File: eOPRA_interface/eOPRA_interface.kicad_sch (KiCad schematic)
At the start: 23 parts, among them J1 CONN_01X02_MALE, J2 CONN_01X04_MALE, J3 CONN_01X04_MALE, J4 CONN_01X02_MALE, J5 CONN_01X03_MALE, J7 header_01x02, J8 CONN_01X04_MALE, Q4 Q_PMOS_DGS, U1 ARM-SWD-10, U10 USB_C_2.0, U27 Mounting-holes, U28 Mounting-holes, U5 XT-X, U7 Mounting-holes, U8 Mounting-holes

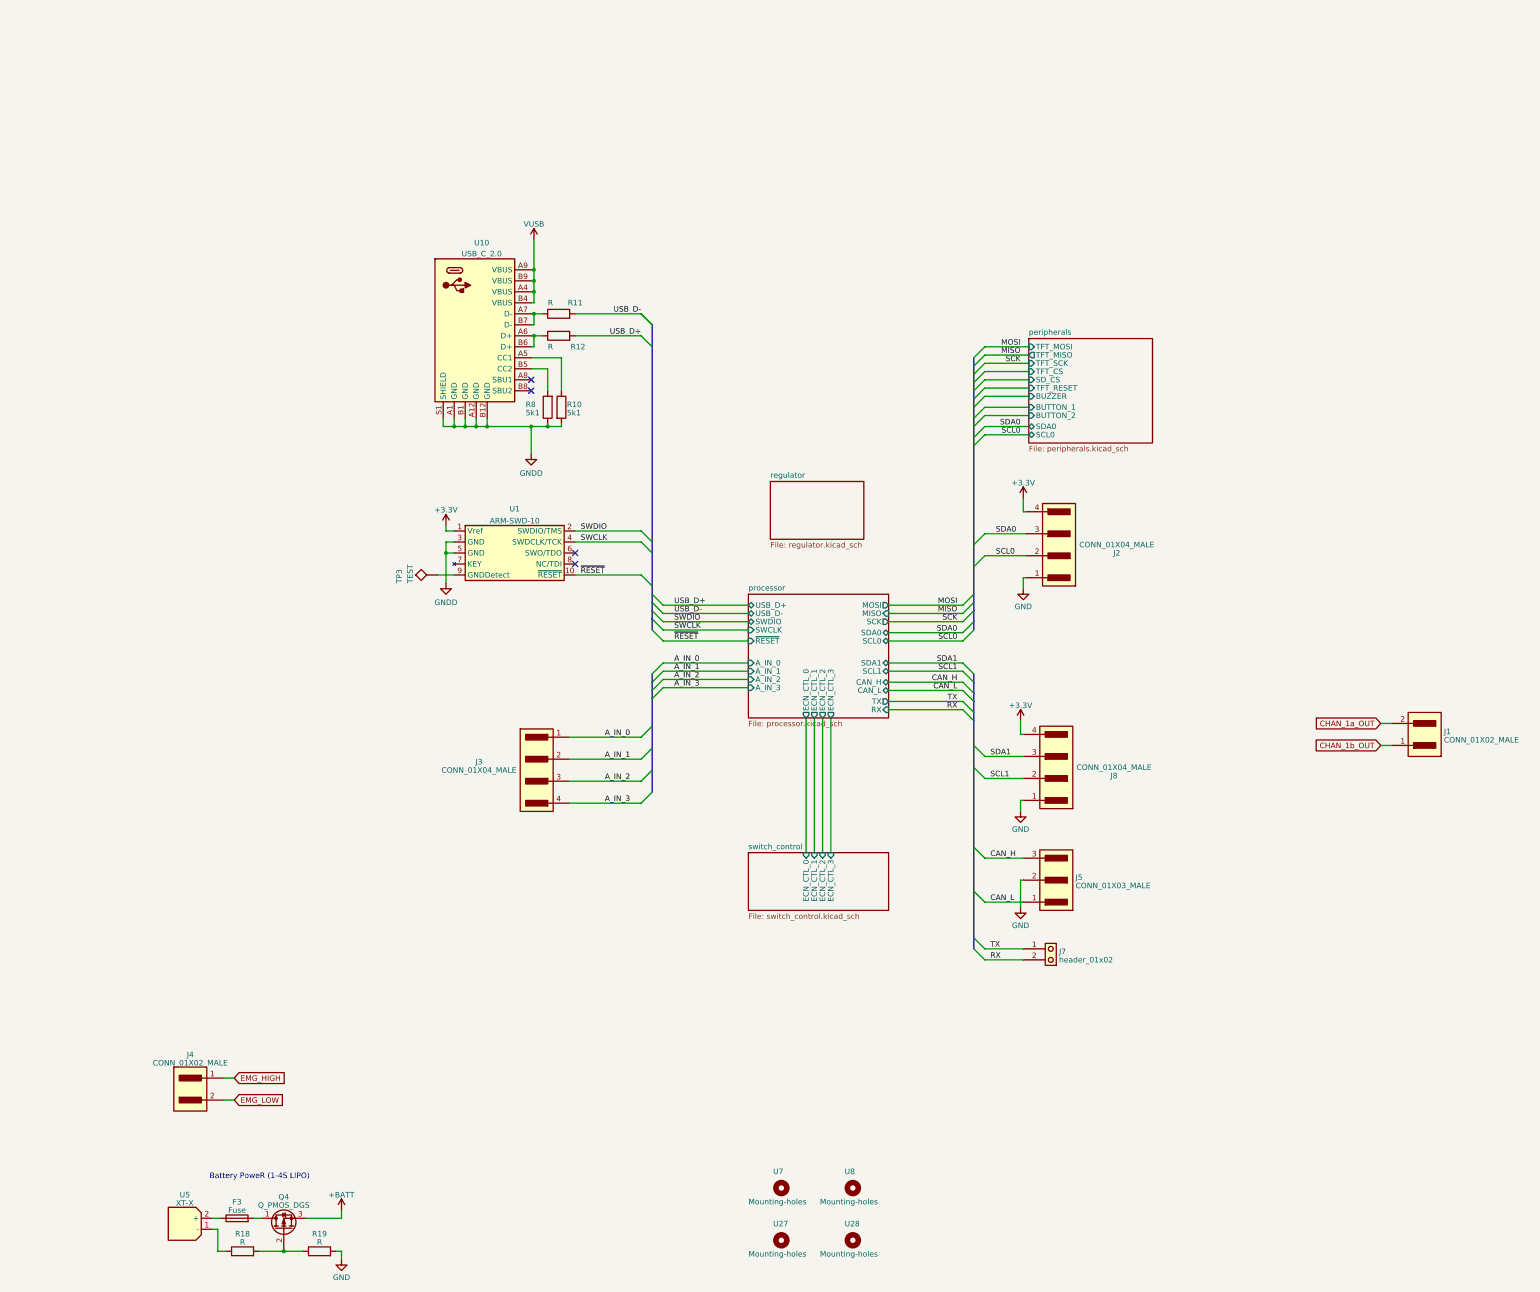
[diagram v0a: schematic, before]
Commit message: schematic v1.0 finished
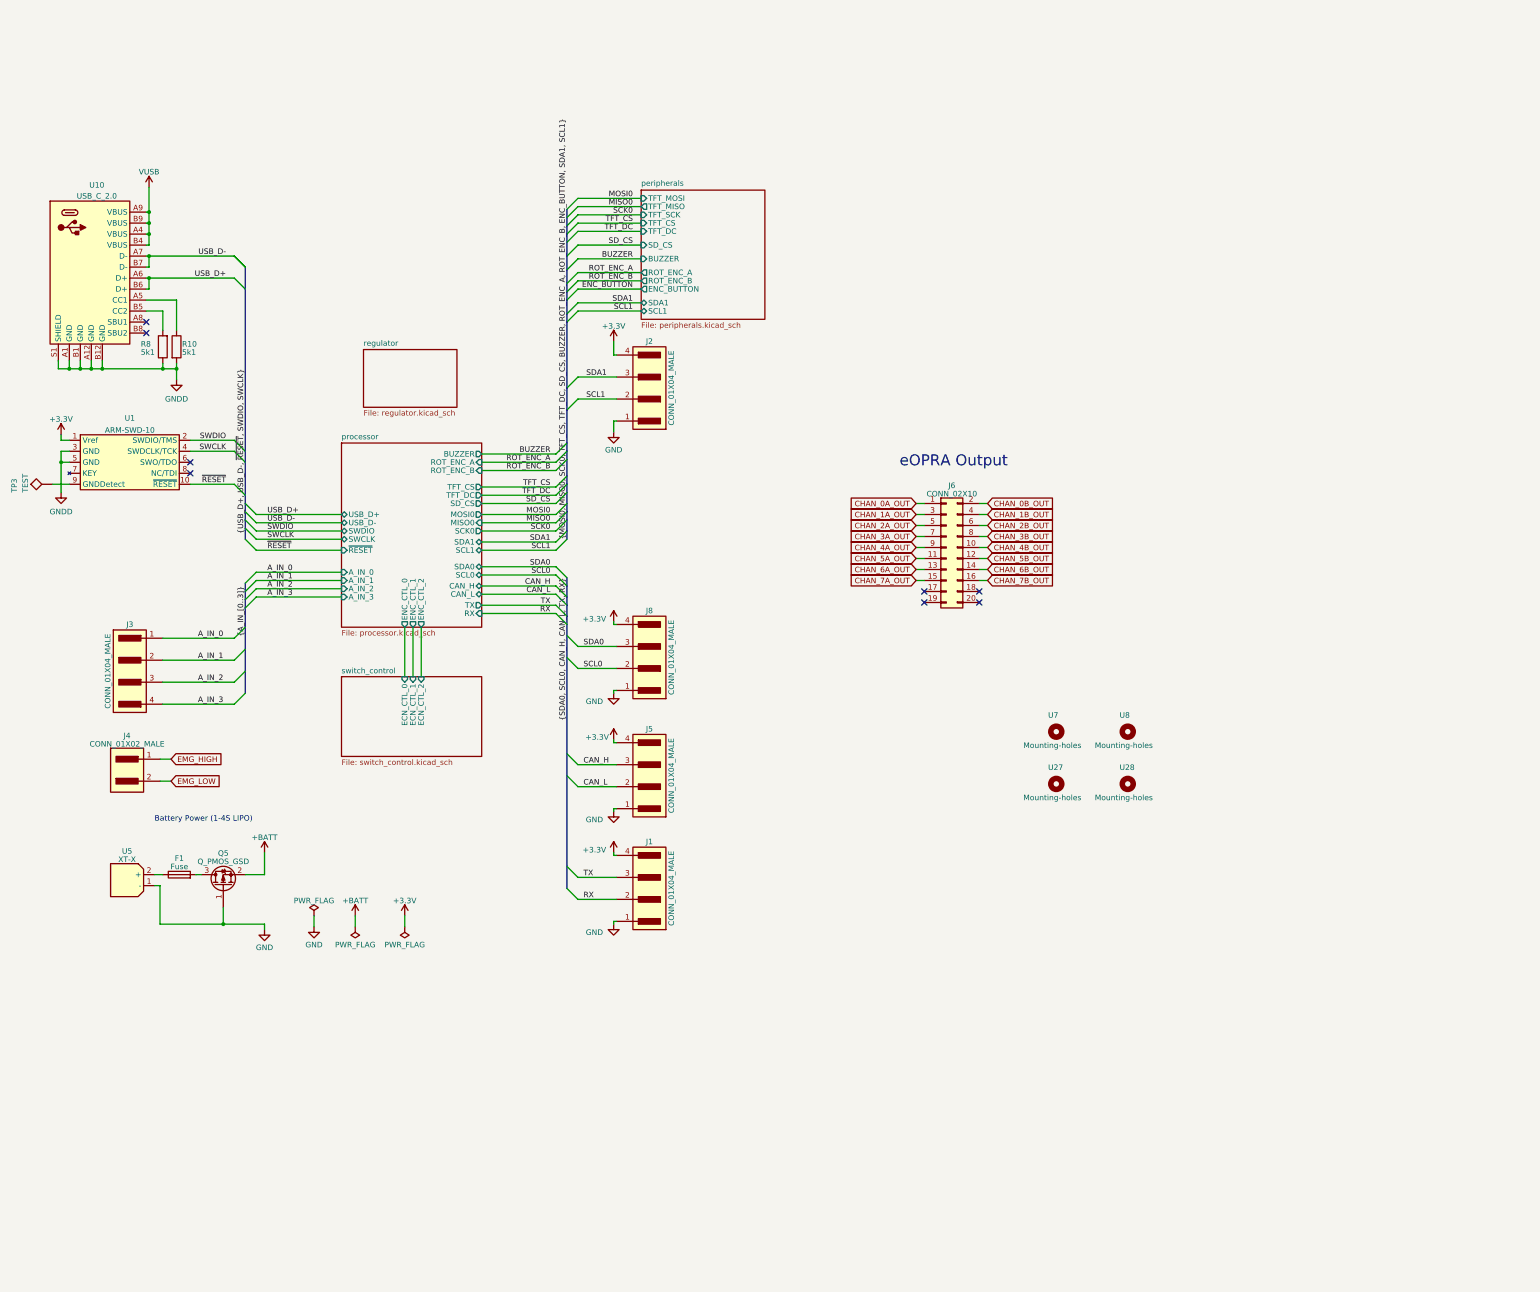
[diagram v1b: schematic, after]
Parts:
- removed F3: Fuse, symbol 4.power.circuitProtection:Fuse
- removed J1: CONN_01X02_MALE, symbol 5.connector.interconnect:CONN_01X02_MALE
- removed J5: CONN_01X03_MALE, symbol 5.connector.interconnect:CONN_01X03_MALE
- removed J7: header_01x02, symbol 5.connector.interconnect:header_01x02
- removed Q4: Q_PMOS_DGS, symbol 1.semi.discrete:Q_PMOS_DGS
- removed R11, R12, R18, R19: R, symbol 2.passive:R
- added F1: Fuse, project_footprints:PTC, symbol 4.power.circuitProtection:Fuse
- added J1, J5: CONN_01X04_MALE, project_footprints:JST_SM04B-GHS-TB(LF)(SN)-, symbol 5.connector.interconnect:CONN_01X04_MALE
- added J6: CONN_02X10, project_footprints:MOLEX_2035642017, symbol 5.connector.interconnect:CONN_02X10
- added Q5: Q_PMOS_GSD, 1_Semi_TO_SOT:TO-252-2, symbol 1.semi.discrete:Q_PMOS_GSD
- J2, J3, J8: footprint (none) -> project_footprints:JST_SM04B-GHS-TB(LF)(SN)-
- J4: footprint (none) -> project_footprints:JST_SM02B_GHS_TB
- R10, R8: PN 1,12 -> (none)
- U1: Link https://www.digikey.com/en/products/detail/samtec-inc/FTSH-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 -> (none); PN 5,5 -> (none)
- U10: PN 5,9 -> (none)
- U5: footprint (none) -> project_footprints:AMASS_XT30PW-M
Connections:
- net +3V3: now also J1.4, J5.4
- net +BATT: now also Q5.2 (S)
- net CAN_H: now also J5.3
- net CAN_L: now also J5.2
- net GND: now also U5.1 (-), J1.1, J5.1, Q5.1 (G)
- net RX: now also J1.2
- net SCL0: now also J8.2; no longer J2.2
- net SCL1: now also J2.2; no longer J8.2
- net SDA0: now also J8.3; no longer J2.3
- net SDA1: now also J2.3; no longer J8.3
- net TX: now also J1.3
- net USB_D+: now also U10.A6 (D+), U10.B6 (D+)
- net USB_D-: now also U10.A7 (D-), U10.B7 (D-)
- net at U5.2 (+): now also F1.1
- new net: F1.2, Q5.3 (D)
- new net CHAN_0A_OUT: J6.1 (P1)
- new net CHAN_0B_OUT: J6.2 (P2)
- new net CHAN_1A_OUT: J6.3 (P3)
- new net CHAN_1B_OUT: J6.4 (P4)
- new net CHAN_2A_OUT: J6.5 (P5)
- new net CHAN_2B_OUT: J6.6 (P6)
- new net CHAN_3A_OUT: J6.7 (P7)
- new net CHAN_3B_OUT: J6.8 (P8)
- new net CHAN_4A_OUT: J6.9 (P9)
- new net CHAN_4B_OUT: J6.10 (P10)
- new net CHAN_5A_OUT: J6.11 (P11)
- new net CHAN_5B_OUT: J6.12 (P12)
- new net CHAN_6A_OUT: J6.13 (P13)
- new net CHAN_6B_OUT: J6.14 (P14)
- new net CHAN_7A_OUT: J6.15 (P15)
- new net CHAN_7B_OUT: J6.16 (P16)
- no-connect marks 4 -> 8
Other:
- sheet peripherals ports: added ENC_BUTTON, ROT_ENC_A, ROT_ENC_B, SCL1, SDA1, TFT_DC; removed BUTTON_1, BUTTON_2, SCL0, SDA0, TFT_RESET
- sheet processor ports: added BUZZER, ENC_CTL_0, ENC_CTL_1, ENC_CTL_2, MISO0, MOSI0, ROT_ENC_A, ROT_ENC_B, SCK0, SD_CS, TFT_CS, TFT_DC; removed ECN_CTL_0, ECN_CTL_1, ECN_CTL_2, ECN_CTL_3, MISO, MOSI, SCK
- sheet switch_control ports: added none; removed ECN_CTL_3
- note added: "Battery Power (1-4S LIPO)"
- note added: "eOPRA Output"
- note removed: "Battery PoweR (1-4S LIPO)"
- moved on the sheet: J4, J8, R10, R8, TP3, U1, U10, U27, U28, U5, U7, U8

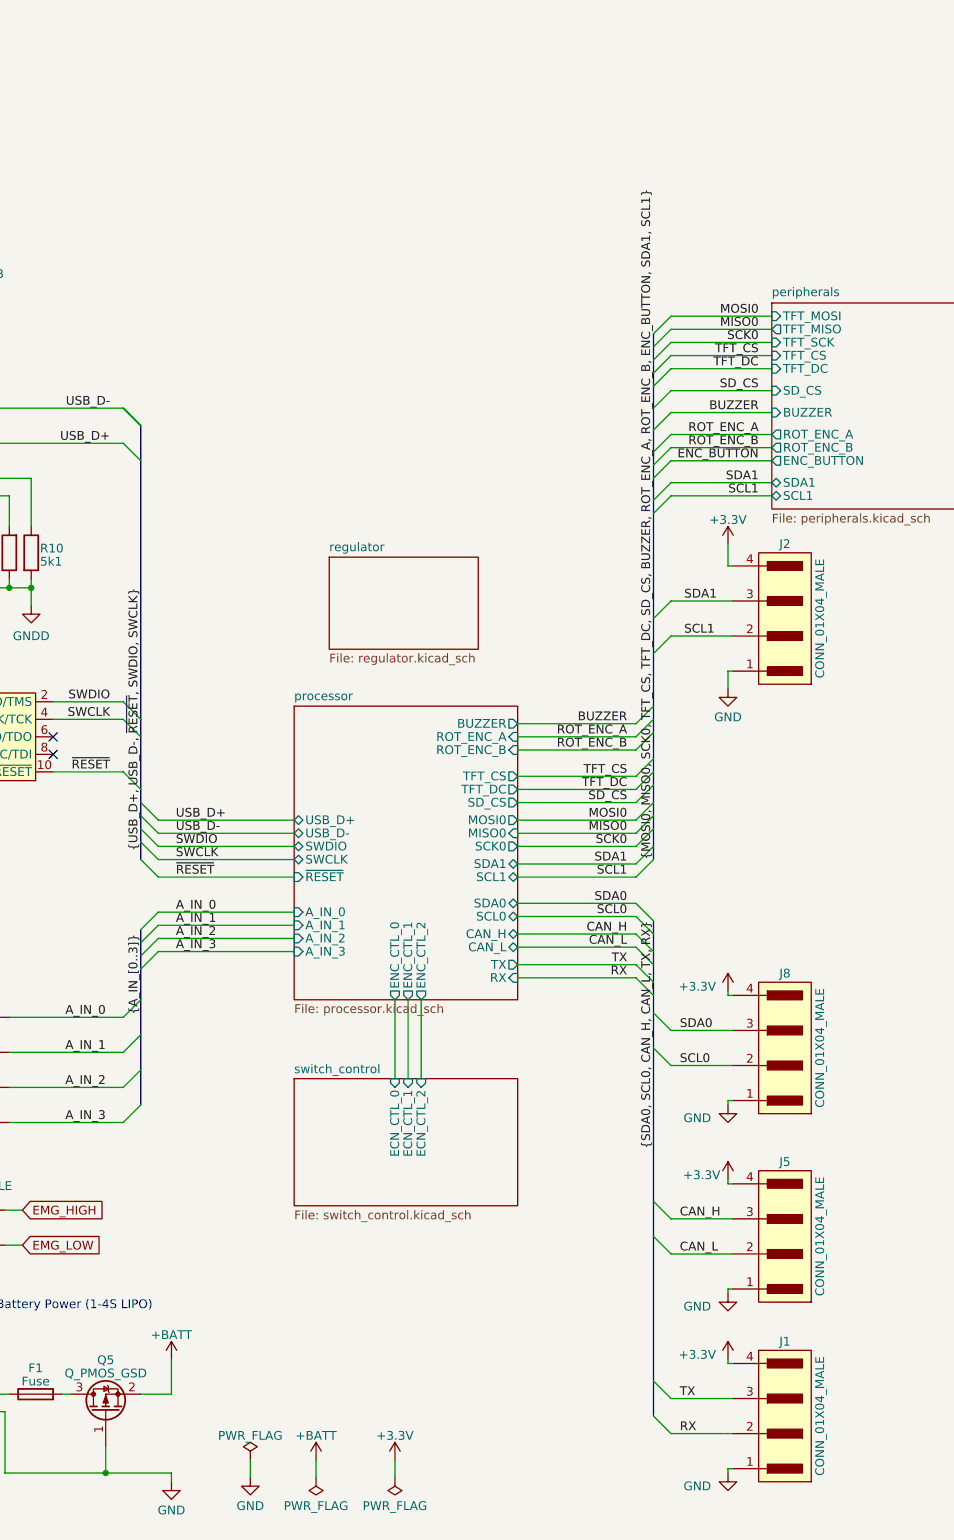
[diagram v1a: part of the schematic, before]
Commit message: Version updates
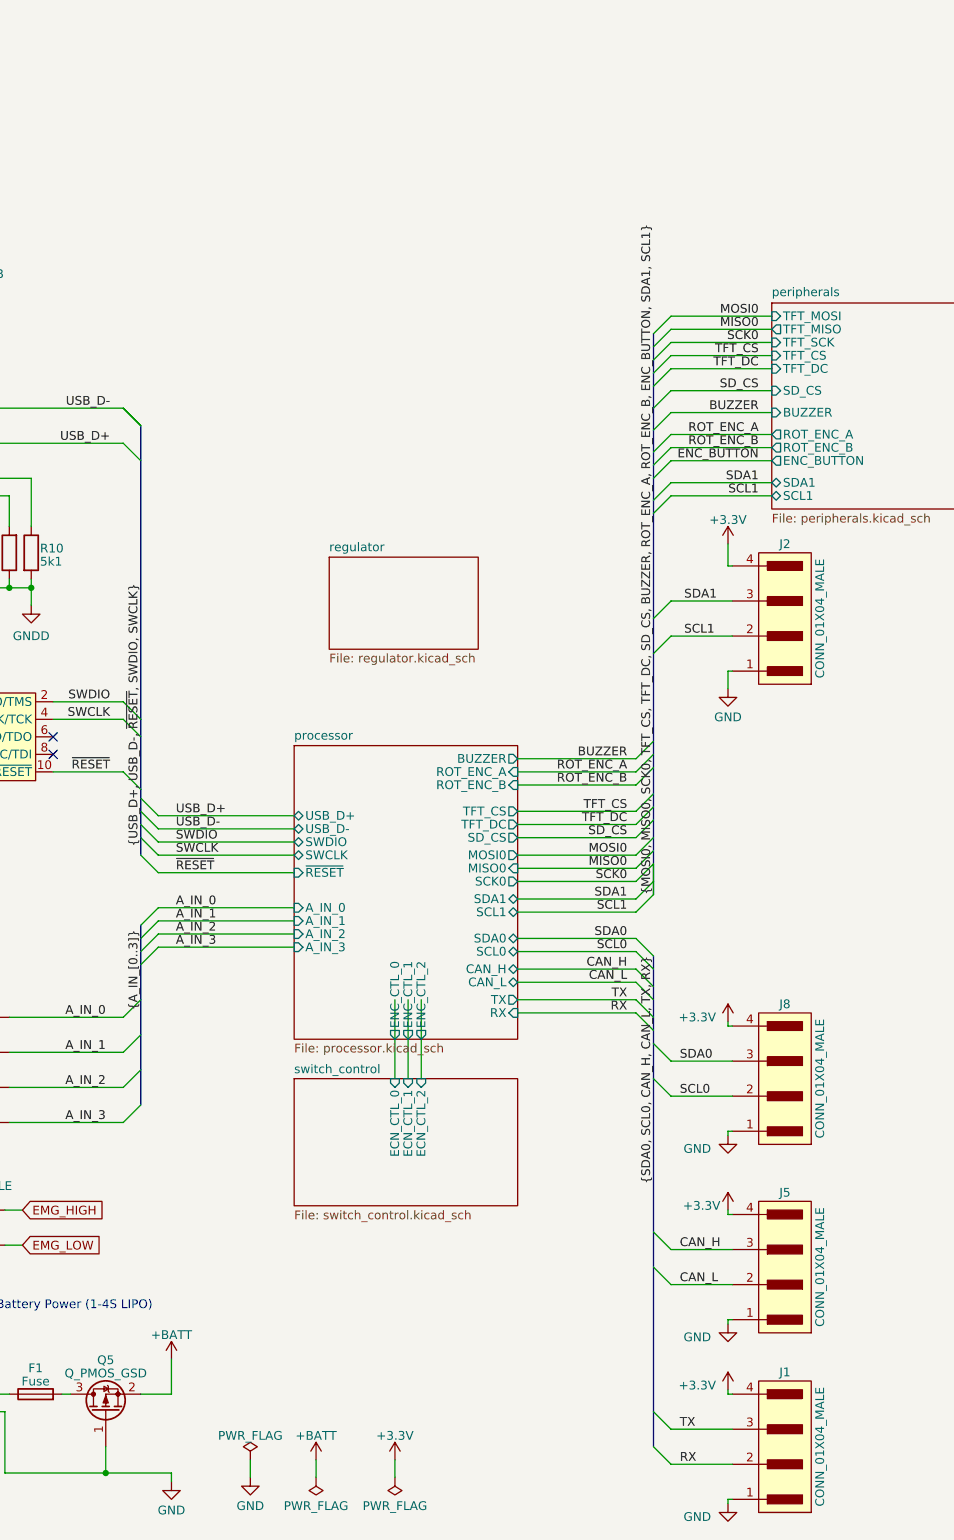
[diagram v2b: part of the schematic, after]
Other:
- company: (none) -> Massachusetts Institute of Technology / MIT Media Lab
- title: (none) -> eOPRA Switch / Stimulation Controller
- moved on the sheet: J1, J5, J8
